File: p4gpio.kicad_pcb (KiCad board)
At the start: 4 copper layers, 87.9 x 23 mm, 94 parts, among them J1 C2760486, J10 Conn_01x04_Socket, J11 Conn_01x04, J2 C2760486, J3 Conn_01x08_Pin, J4 Conn_01x08_Pin, J5 Conn_01x08_Pin, J6 Conn_01x08_Pin, J7 Conn_01x08_Pin, J8 Conn_01x08_Pin, J9 Conn_01x04_Socket, Q1 MBT3906DW1, Q2 AO3401A, Q3 MBT3906DW1, Q4 AO3401A, U1 TLV62569DBV, U3 W25Q128JVS, U4 TLV62569DBV, Y1 40MHz(+-10 ppm) C501798

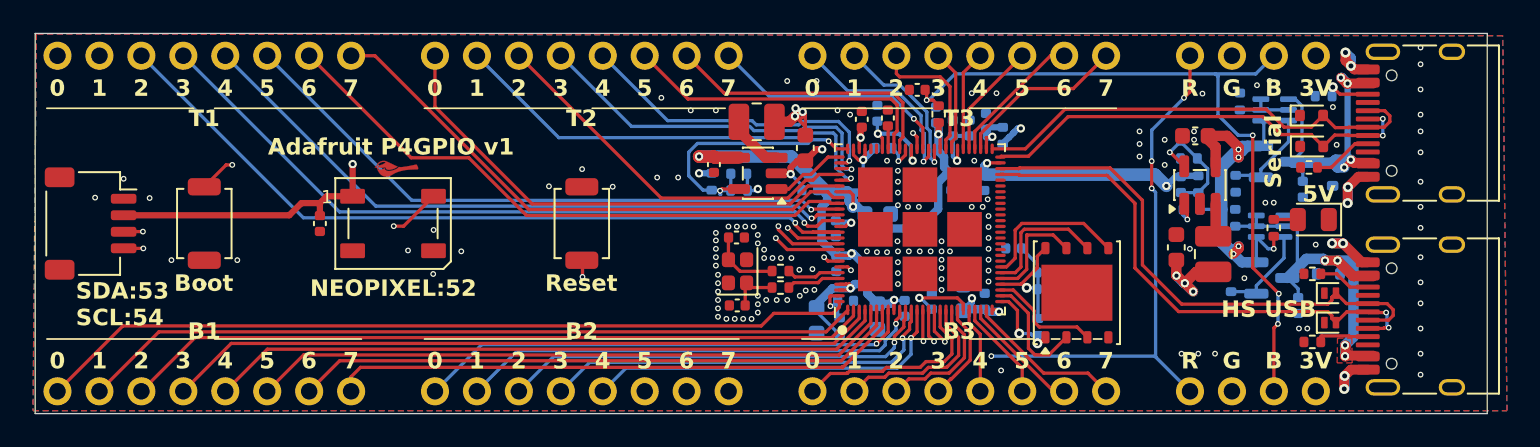
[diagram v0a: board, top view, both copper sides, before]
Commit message: Ordered
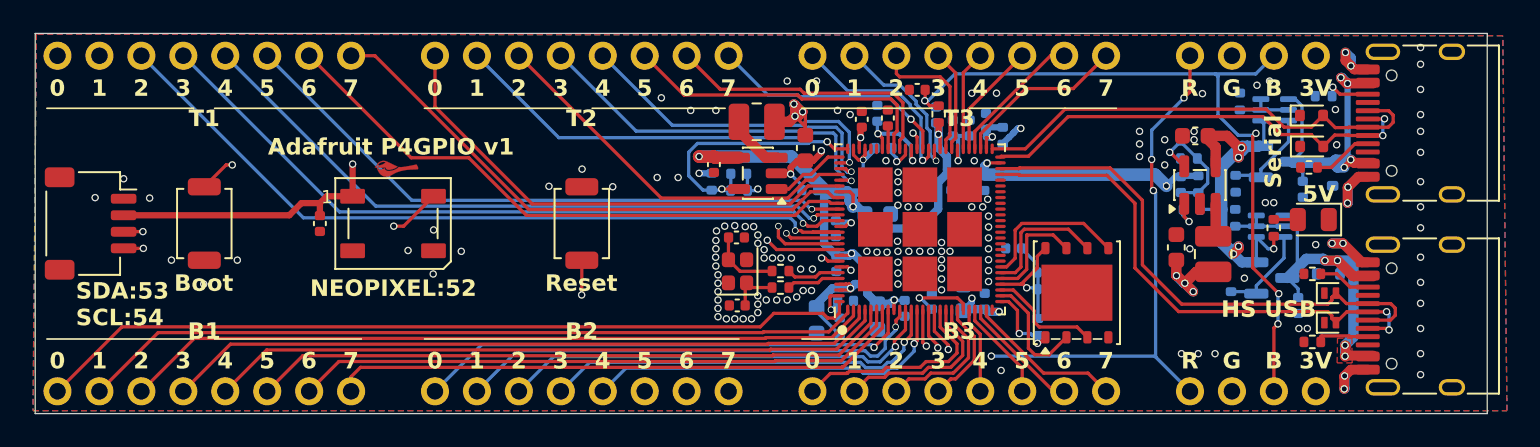
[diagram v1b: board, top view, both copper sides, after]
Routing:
- net /Minimal P4 V3/VDD_HP: track 56.3 -> 58.7 mm
- net /B2_5: track 20.1 -> 21.5 mm
- net /RESET: track 64.7 -> 65.4 mm
- net /BOOT: track 94.8 -> 95.5 mm
- net /B2_7: track 16.5 -> 17.1 mm
